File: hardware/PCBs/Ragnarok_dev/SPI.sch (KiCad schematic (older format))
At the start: 5 parts

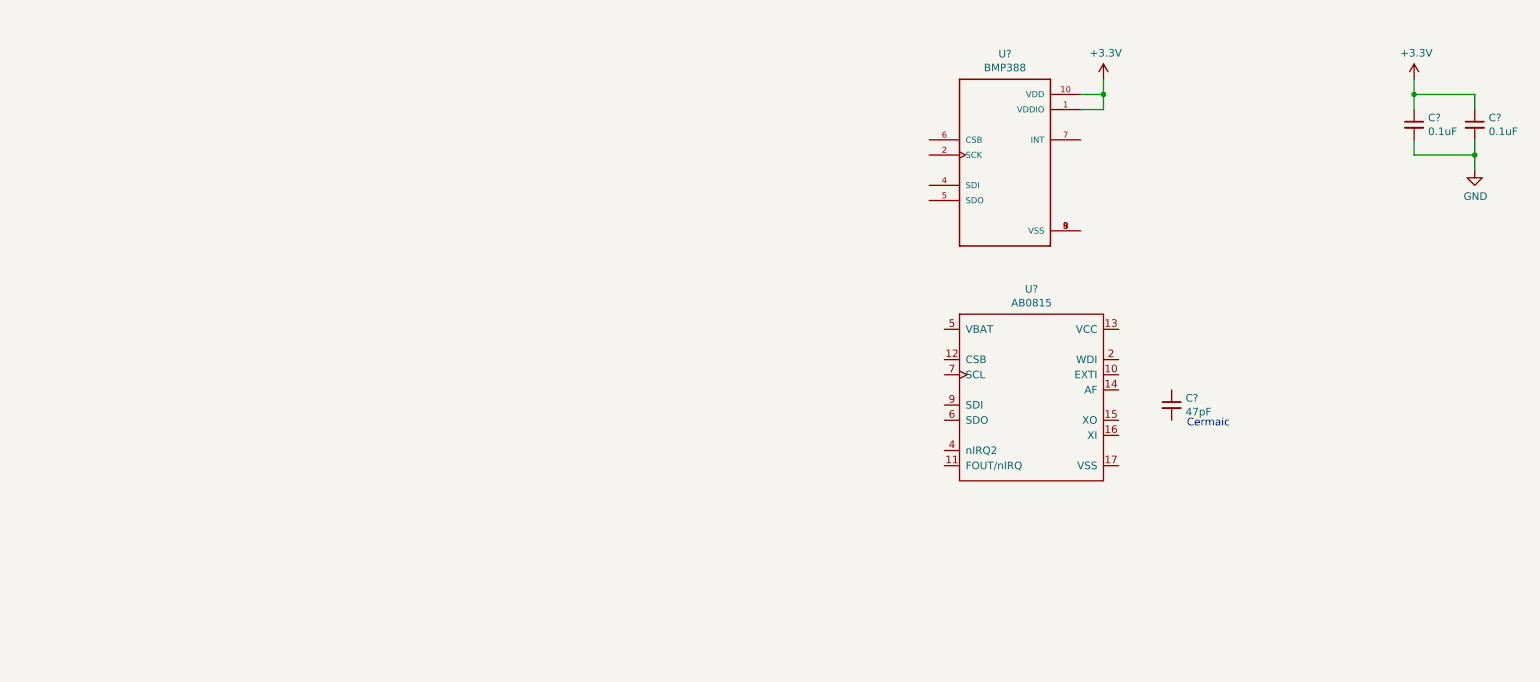
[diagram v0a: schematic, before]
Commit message: Update
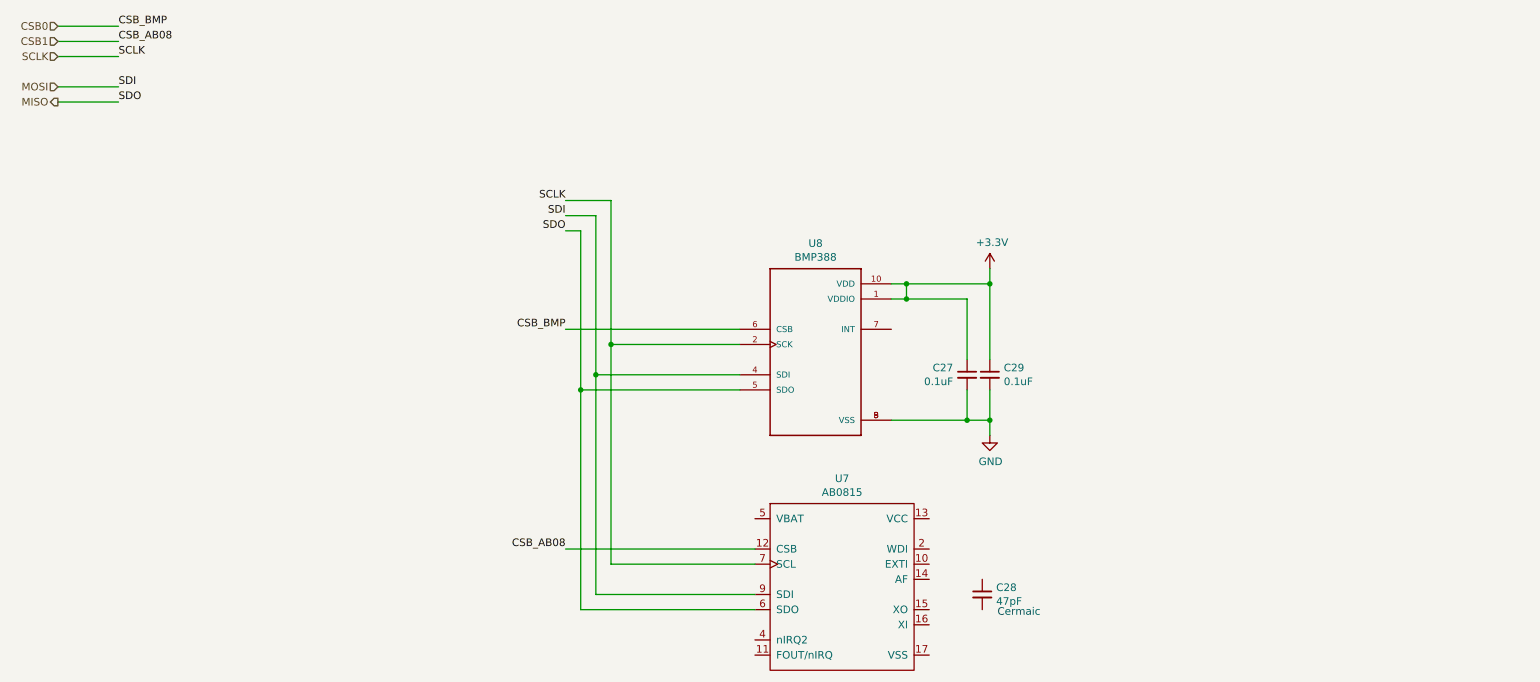
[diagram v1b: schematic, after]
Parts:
- gave numbers to parts that had none: 5
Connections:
- net GND: now also U8.3 (VSS), U8.8 (VSS), U8.9 (VSS)
- net SCLK: now reaches U8.2 (SCK)
- net SCLK: now also U7.7 (SCL)
- net MOSI: now reaches U8.4 (SDI)
- net MOSI: now also U7.9 (SDI)
- net MISO: now reaches U8.5 (SDO)
- net MISO: now also U7.6 (SDO)
- net CSB0: now reaches U8.6 (CSB)
- net CSB1: now reaches U7.12 (CSB)
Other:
- moved on the sheet: C27, C28, C29, U7, U8
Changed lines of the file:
@@
 $Descr A4 11693 8268
 encoding utf-8
-Sheet 3 3
+Sheet 3 4
 Title ""
 Date ""
@@
 $EndDescr
 $Comp
-L Device:C_Small C?
+L Device:C_Small C29
+U 1 1 5E1A3CEA
+P 7500 3400
+F 0 "C29" H 7592 3446 50  0000 L CNN
+F 1 "0.1uF" H 7592 3355 50  0000 L CNN
+F 2 "" H 7500 3400 50  0001 C CNN
+F 3 "~" H 7500 3400 50  0001 C CNN
+	1    7500 3400
+	1    0    0    -1
+$EndComp
+$Comp
+L power:+3.3V #PWR0117
+U 1 1 5E1AEFA0
+P 7500 2700
+F 0 "#PWR0117" H 7500 2550 50  0001 C CNN
+F 1 "+3.3V" H 7515 2873 50  0000 C CNN
+F 2 "" H 7500 2700 50  0001 C CNN
+F 3 "" H 7500 2700 50  0001 C CNN
+	1    7500 2700
+	1    0    0    -1
+$EndComp
+$Comp
+L BMP388:BMP388 U8
+U 1 1 5E1A1175
+P 6350 3300
+F 0 "U8" H 6350 4067 50  0000 C CNN
+F 1 "BMP388" H 6350 3976 50  0000 C CNN
+F 2 "PQFN50P200X200X80-10N" H 6350 3300 50  0001 L BNN
+F 3 "BOSCH" H 6350 3300 50  0001 L BNN
+F 4 "1.1" H 6350 3300 50  0001 L BNN "Field4"
+F 5 "IPC 7351B" H 6350 3300 50  0001 L BNN "Field5"
+	1    6350 3300
+	1    0    0    -1
+$EndComp
+$Comp
+L AB0815:AB0815 U7
+U 1 1 5E1B97AD
+P 5650 4400
+F 0 "U7" H 6525 4715 50  0000 C CNN
+F 1 "AB0815" H 6525 4624 50  0000 C CNN
+F 2 "" H 6550 4600 50  0001 C CNN
+F 3 "" H 6550 4600 50  0001 C CNN
+	1    5650 4400
+	1    0    0    -1
+$EndComp
+$Comp
+L Device:C_Small C28
+U 1 1 5E1BCE97
+P 7450 4850
+F 0 "C28" H 7542 4896 50  0000 L CNN
+F 1 "47pF" H 7542 4805 50  0000 L CNN
+F 2 "" H 7450 4850 50  0001 C CNN
+F 3 "~" H 7450 4850 50  0001 C CNN
+	1    7450 4850
+	1    0    0    -1
+$EndComp
+Text Notes 7550 5000 0    50   ~ 0
+Cermaic\n
+$Comp
+L Device:C_Small C27
 U 1 1 5E1A3829
-P 10300 1750
-F 0 "C?" H 10392 1796 50  0000 L CNN
-F 1 "0.1uF" H 10392 1705 50  0000 L CNN
-F 2 "" H 10300 1750 50  0001 C CNN
-F 3 "~" H 10300 1750 50  0001 C CNN
-	1    10300 1750
-	1    0    0    -1
-$EndComp
-$Comp
-L Device:C_Small C?
-U 1 1 5E1A3CEA
-P 10700 1750
-F 0 "C?" H 10792 1796 50  0000 L CNN
-F 1 "0.1uF" H 10792 1705 50  0000 L CNN
-F 2 "" H 10700 1750 50  0001 C CNN
-F 3 "~" H 10700 1750 50  0001 C CNN
-	1    10700 1750
-	1    0    0    -1
-$EndComp
-$Comp
-L power:+3.3V #PWR?
-U 1 1 5E1A68CE
-P 10300 1450
-F 0 "#PWR?" H 10300 1300 50  0001 C CNN
-F 1 "+3.3V" H 10315 1623 50  0000 C CNN
-F 2 "" H 10300 1450 50  0001 C CNN
-F 3 "" H 10300 1450 50  0001 C CNN
-	1    10300 1450
-	1    0    0    -1
-$EndComp
-$Comp
-L power:GND #PWR?
-U 1 1 5E1A7831
-P 10700 2050
-F 0 "#PWR?" H 10700 1800 50  0001 C CNN
-F 1 "GND" H 10705 1877 50  0000 C CNN
-F 2 "" H 10700 2050 50  0001 C CNN
-F 3 "" H 10700 2050 50  0001 C CNN
-	1    10700 2050
-	1    0    0    -1
-$EndComp
-Wire Wire Line
-	10300 1450 10300 1550
-Wire Wire Line
-	10300 1550 10700 1550
-Wire Wire Line
-	10700 1550 10700 1650
-Connection ~ 10300 1550
-Wire Wire Line
-	10300 1550 10300 1650
-Wire Wire Line
-	8250 1650 8100 1650
-Wire Wire Line
-	8250 1550 8100 1550
-Wire Wire Line
-	10300 1850 10300 1950
-Wire Wire Line
-	10300 1950 10700 1950
-Wire Wire Line
-	10700 1950 10700 2050
-Wire Wire Line
-	10700 1850 10700 1950
-Connection ~ 10700 1950
-$Comp
-L power:+3.3V #PWR?
-U 1 1 5E1AEFA0
-P 8250 1450
-F 0 "#PWR?" H 8250 1300 50  0001 C CNN
-F 1 "+3.3V" H 8265 1623 50  0000 C CNN
-F 2 "" H 8250 1450 50  0001 C CNN
-F 3 "" H 8250 1450 50  0001 C CNN
-	1    8250 1450
-	1    0    0    -1
-$EndComp
-Wire Wire Line
-	8250 1450 8250 1550
-Connection ~ 8250 1550
-Wire Wire Line
-	8250 1550 8250 1650
-$Comp
-L BMP388:BMP388 U?
-U 1 1 5E1A1175
-P 7600 2050
-F 0 "U?" H 7600 2817 50  0000 C CNN
-F 1 "BMP388" H 7600 2726 50  0000 C CNN
-F 2 "PQFN50P200X200X80-10N" H 7600 2050 50  0001 L BNN
-F 3 "BOSCH" H 7600 2050 50  0001 L BNN
-F 4 "1.1" H 7600 2050 50  0001 L BNN "Field4"
-F 5 "IPC 7351B" H 7600 2050 50  0001 L BNN "Field5"
-	1    7600 2050
-	1    0    0    -1
-$EndComp
-$Comp
-L AB0815:AB0815 U?
-U 1 1 5E1B97AD
-P 6900 3150
-F 0 "U?" H 7775 3465 50  0000 C CNN
-F 1 "AB0815" H 7775 3374 50  0000 C CNN
-F 2 "" H 7800 3350 50  0001 C CNN
-F 3 "" H 7800 3350 50  0001 C CNN
-	1    6900 3150
-	1    0    0    -1
-$EndComp
-$Comp
-L Device:C_Small C?
-U 1 1 5E1BCE97
-P 8700 3600
-F 0 "C?" H 8792 3646 50  0000 L CNN
-F 1 "47pF" H 8792 3555 50  0000 L CNN
-F 2 "" H 8700 3600 50  0001 C CNN
-F 3 "~" H 8700 3600 50  0001 C CNN
-	1    8700 3600
-	1    0    0    -1
-$EndComp
-Text Notes 8800 3750 0    50   ~ 0
-Cermaic\n
+P 7350 3400
+F 0 "C27" H 7442 3446 50  0000 L CNN
+F 1 "0.1uF" H 7442 3355 50  0000 L CNN
+F 2 "" H 7350 3400 50  0001 C CNN
+F 3 "~" H 7350 3400 50  0001 C CNN
+	1    7350 3400
+	-1   0    0    -1
+$EndComp
+Wire Wire Line
+	7500 2700 7500 2800
+Wire Wire Line
+	7500 2800 6950 2800
+Wire Wire Line
+	6850 2900 6950 2900
+Wire Wire Line
+	6950 2900 6950 2800
+Connection ~ 6950 2800
+Wire Wire Line
+	6950 2800 6850 2800
+Wire Wire Line
+	7350 2900 7350 3300
+Wire Wire Line
+	7350 3500 7350 3700
+Wire Wire Line
+	7500 2800 7500 3300
+Connection ~ 7500 2800
+Wire Wire Line
+	7500 3500 7500 3700
+Wire Wire Line
+	7500 3700 7350 3700
+$Comp
+L power:GND #PWR0118
+U 1 1 5E2332D8
+P 7500 3800
+F 0 "#PWR0118" H 7500 3550 50  0001 C CNN
+F 1 "GND" H 7505 3627 50  0000 C CNN
+F 2 "" H 7500 3800 50  0001 C CNN
+F 3 "" H 7500 3800 50  0001 C CNN
+	1    7500 3800
+	1    0    0    -1
+$EndComp
+Wire Wire Line
+	7500 3700 7500 3800
+Connection ~ 7500 3700
+Wire Wire Line
+	5000 3200 5000 4650
+Wire Wire Line
+	4900 3400 4900 4850
+Wire Wire Line
+	4800 3500 4800 4950
+Wire Wire Line
+	5000 3200 5000 2250
+Connection ~ 5000 3200
+Wire Wire Line
+	4900 3400 4900 2350
+Connection ~ 4900 3400
+Wire Wire Line
+	4800 3500 4800 2450
+Connection ~ 4800 3500
+Text Label 4700 2250 2    50   ~ 0
+SCLK
+Text Label 4700 2350 2    50   ~ 0
+SDI
+Text Label 4700 2450 2    50   ~ 0
+SDO
+Wire Wire Line
+	4800 2450 4700 2450
+Wire Wire Line
+	4700 2350 4900 2350
+Wire Wire Line
+	4700 2250 5000 2250
+Text HLabel 1350 1300 0    50   Input ~ 0
+SCLK
+Text HLabel 1350 1500 0    50   Input ~ 0
+MOSI
+Text HLabel 1350 1600 0    50   Output ~ 0
+MISO
+Text Label 1750 1300 0    50   ~ 0
+SCLK
+Text Label 1750 1500 0    50   ~ 0
+SDI
+Text Label 1750 1600 0    50   ~ 0
+SDO
+Wire Wire Line
+	1350 1300 1750 1300
+Wire Wire Line
+	1350 1500 1750 1500
+Wire Wire Line
+	1350 1600 1750 1600
+Text HLabel 1350 1100 0    50   Input ~ 0
+CSB0
+Text HLabel 1350 1200 0    50   Input ~ 0
+CSB1
+Text Label 1750 1100 0    50   ~ 0
+CSB_BMP
+Text Label 1750 1200 0    50   ~ 0
+CSB_AB08
+Wire Wire Line
+	1350 1200 1750 1200
+Wire Wire Line
+	1350 1100 1750 1100
+Text Label 4700 3100 2    50   ~ 0
+CSB_BMP
+Text Label 4700 4550 2    50   ~ 0
+CSB_AB08
+Connection ~ 7350 3700
+Wire Wire Line
+	6850 3700 7350 3700
+Wire Wire Line
+	6950 2900 7350 2900
+Connection ~ 6950 2900
+Wire Wire Line
+	4700 4550 5950 4550
+Wire Wire Line
+	5000 4650 5950 4650
+Wire Wire Line
+	4900 4850 5950 4850
+Wire Wire Line
+	4800 4950 5950 4950
+Wire Wire Line
+	4700 3100 5850 3100
+Wire Wire Line
+	5000 3200 5850 3200
+Wire Wire Line
+	4900 3400 5850 3400
+Wire Wire Line
+	4800 3500 5850 3500
 $EndSCHEMATC
